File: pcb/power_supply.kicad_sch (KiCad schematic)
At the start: 16 parts, among them IC1 TLV76150DCYR, IC2 LM3940IMP-3.3_NOPB, J1 Jack-DC

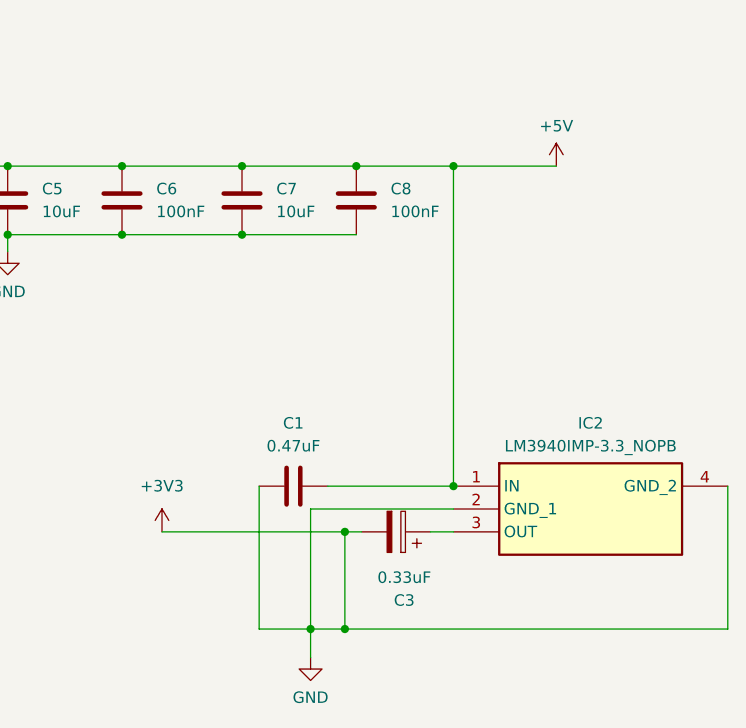
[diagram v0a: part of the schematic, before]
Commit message: a lot of audio finished, now onto ui
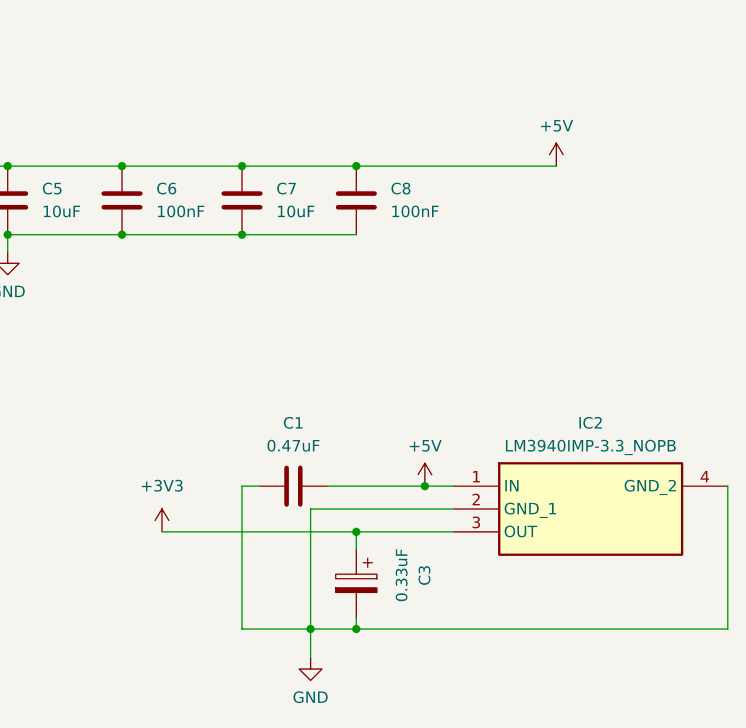
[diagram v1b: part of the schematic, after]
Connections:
- net +3V3: now also C3.1, IC2.3 (OUT); no longer C1.1, C2.2, C3.2, C4.2, C5.2, C6.2, C64.2, C65.2, C66.2, C67.2, C7.2, C8.2, IC1.1 (GND), IC2.2 (GND_1), IC2.4 (GND_2), J1.2
- new net GND: C1.1, C2.2, C3.2, C4.2, C5.2, C6.2, C64.2, C65.2, C66.2, C67.2, C7.2, C8.2, IC1.1 (GND), IC2.2 (GND_1), IC2.4 (GND_2), J1.2
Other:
- moved on the sheet: C3
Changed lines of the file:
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@@
   (junction (at 92.71 100.965) (diameter 0) (color 0 0 0 0)
   )
-  (junction (at 193.04 107.315) (diameter 0) (color 0 0 0 0)
-  )
-  (junction (at 205.105 55.88) (diameter 0) (color 0 0 0 0)
-  )
   (junction (at 92.71 50.8) (diameter 0) (color 0 0 0 0)
   )
@@
   (junction (at 189.23 107.315) (diameter 0) (color 0 0 0 0)
   )
+  (junction (at 194.31 107.315) (diameter 0) (color 0 0 0 0)
+  )
   (junction (at 181.61 55.88) (diameter 0) (color 0 0 0 0)
   )
@@
   (junction (at 80.01 93.345) (diameter 0) (color 0 0 0 0)
   )
-  (junction (at 193.04 96.52) (diameter 0) (color 0 0 0 0)
-  )
   (junction (at 155.575 63.5) (diameter 0) (color 0 0 0 0)
   )
   (junction (at 168.275 63.5) (diameter 0) (color 0 0 0 0)
   )
-  (junction (at 205.105 91.44) (diameter 0) (color 0 0 0 0)
-  )
   (junction (at 102.235 50.8) (diameter 0) (color 0 0 0 0)
   )
@@
   (junction (at 102.235 39.37) (diameter 0) (color 0 0 0 0)
   )
+  (junction (at 201.93 91.44) (diameter 0) (color 0 0 0 0)
+  )
+  (junction (at 194.31 96.52) (diameter 0) (color 0 0 0 0)
+  )
   (junction (at 155.575 55.88) (diameter 0) (color 0 0 0 0)
   )
@@
     (stroke (width 0) (type default))
   )
-  (wire (pts (xy 183.515 107.315) (xy 189.23 107.315))
+  (wire (pts (xy 172.72 96.52) (xy 194.31 96.52))
+    (stroke (width 0) (type default))
+  )
+  (wire (pts (xy 181.61 107.315) (xy 189.23 107.315))
     (stroke (width 0) (type default))
   )
@@
     (stroke (width 0) (type default))
   )
-  (wire (pts (xy 172.72 96.52) (xy 193.04 96.52))
-    (stroke (width 0) (type default))
-  )
-  (wire (pts (xy 191.135 91.44) (xy 205.105 91.44))
+  (wire (pts (xy 191.135 91.44) (xy 201.93 91.44))
     (stroke (width 0) (type default))
   )
@@
     (stroke (width 0) (type default))
   )
-  (wire (pts (xy 202.565 96.52) (xy 205.105 96.52))
+  (wire (pts (xy 201.93 91.44) (xy 205.105 91.44))
     (stroke (width 0) (type default))
   )
@@
     (stroke (width 0) (type default))
   )
-  (wire (pts (xy 189.23 107.315) (xy 193.04 107.315))
-    (stroke (width 0) (type default))
-  )
   (wire (pts (xy 80.01 93.345) (xy 92.71 93.345))
     (stroke (width 0) (type default))
@@
     (stroke (width 0) (type default))
   )
+  (wire (pts (xy 194.31 106.045) (xy 194.31 107.315))
+    (stroke (width 0) (type default))
+  )
   (wire (pts (xy 92.71 100.965) (xy 106.045 100.965))
     (stroke (width 0) (type default))
@@
     (stroke (width 0) (type default))
   )
+  (wire (pts (xy 194.31 107.315) (xy 235.585 107.315))
+    (stroke (width 0) (type default))
+  )
   (wire (pts (xy 235.585 91.44) (xy 235.585 107.315))
     (stroke (width 0) (type default))
   )
+  (wire (pts (xy 205.105 96.52) (xy 194.31 96.52))
+    (stroke (width 0) (type default))
+  )
   (wire (pts (xy 106.045 93.345) (xy 118.745 93.345))
     (stroke (width 0) (type default))
   )
-  (wire (pts (xy 194.945 96.52) (xy 193.04 96.52))
-    (stroke (width 0) (type default))
-  )
   (wire (pts (xy 66.675 55.88) (xy 69.85 55.88))
     (stroke (width 0) (type default))
   )
-  (wire (pts (xy 194.31 55.88) (xy 205.105 55.88))
+  (wire (pts (xy 194.31 55.88) (xy 216.535 55.88))
+    (stroke (width 0) (type default))
+  )
+  (wire (pts (xy 92.71 93.345) (xy 106.045 93.345))
+    (stroke (width 0) (type default))
+  )
+  (wire (pts (xy 80.01 100.965) (xy 80.01 102.87))
+    (stroke (width 0) (type default))
+  )
+  (wire (pts (xy 92.71 52.705) (xy 92.71 50.8))
+    (stroke (width 0) (type default))
+  )
+  (wire (pts (xy 181.61 63.5) (xy 194.31 63.5))
+    (stroke (width 0) (type default))
+  )
+  (wire (pts (xy 181.61 91.44) (xy 181.61 107.315))
+    (stroke (width 0) (type default))
+  )
+  (wire (pts (xy 102.235 55.88) (xy 102.235 66.675))
+    (stroke (width 0) (type default))
+  )
+  (wire (pts (xy 189.23 107.315) (xy 189.23 110.49))
+    (stroke (width 0) (type default))
+  )
+  (wire (pts (xy 98.425 39.37) (xy 102.235 39.37))
+    (stroke (width 0) (type default))
+  )
+  (wire (pts (xy 168.275 55.88) (xy 181.61 55.88))
+    (stroke (width 0) (type default))
+  )
+  (wire (pts (xy 102.235 48.26) (xy 102.235 50.8))
+    (stroke (width 0) (type default))
+  )
+  (wire (pts (xy 92.71 50.8) (xy 102.235 50.8))
+    (stroke (width 0) (type default))
+  )
+  (wire (pts (xy 135.89 57.785) (xy 135.89 55.88))
     (stroke (width 0) (type default))
   )
@@
     (stroke (width 0) (type default))
   )
-  (wire (pts (xy 92.71 93.345) (xy 106.045 93.345))
-    (stroke (width 0) (type default))
-  )
-  (wire (pts (xy 80.01 100.965) (xy 80.01 102.87))
-    (stroke (width 0) (type default))
-  )
-  (wire (pts (xy 92.71 52.705) (xy 92.71 50.8))
-    (stroke (width 0) (type default))
-  )
-  (wire (pts (xy 181.61 63.5) (xy 194.31 63.5))
-    (stroke (width 0) (type default))
-  )
-  (wire (pts (xy 183.515 91.44) (xy 183.515 107.315))
-    (stroke (width 0) (type default))
-  )
-  (wire (pts (xy 102.235 55.88) (xy 102.235 66.675))
-    (stroke (width 0) (type default))
-  )
-  (wire (pts (xy 189.23 107.315) (xy 189.23 110.49))
-    (stroke (width 0) (type default))
-  )
-  (wire (pts (xy 98.425 39.37) (xy 102.235 39.37))
-    (stroke (width 0) (type default))
-  )
-  (wire (pts (xy 168.275 55.88) (xy 181.61 55.88))
-    (stroke (width 0) (type default))
-  )
-  (wire (pts (xy 102.235 48.26) (xy 102.235 50.8))
-    (stroke (width 0) (type default))
-  )
-  (wire (pts (xy 92.71 50.8) (xy 102.235 50.8))
-    (stroke (width 0) (type default))
-  )
-  (wire (pts (xy 135.89 57.785) (xy 135.89 55.88))
-    (stroke (width 0) (type default))
-  )
   (wire (pts (xy 168.275 63.5) (xy 181.61 63.5))
     (stroke (width 0) (type default))
@@
     (stroke (width 0) (type default))
   )
-  (wire (pts (xy 193.04 107.315) (xy 235.585 107.315))
-    (stroke (width 0) (type default))
-  )
-  (wire (pts (xy 205.105 55.88) (xy 205.105 91.44))
+  (wire (pts (xy 189.23 107.315) (xy 194.31 107.315))
+    (stroke (width 0) (type default))
+  )
+  (wire (pts (xy 181.61 91.44) (xy 183.515 91.44))
+    (stroke (width 0) (type default))
+  )
+  (wire (pts (xy 194.31 96.52) (xy 194.31 98.425))
     (stroke (width 0) (type default))
   )
   (wire (pts (xy 155.575 63.5) (xy 168.275 63.5))
-    (stroke (width 0) (type default))
-  )
-  (wire (pts (xy 193.04 96.52) (xy 193.04 107.315))
-    (stroke (width 0) (type default))
-  )
-  (wire (pts (xy 205.105 55.88) (xy 216.535 55.88))
     (stroke (width 0) (type default))
   )
@@
         (path "/eb787481-08cd-41a4-a128-173fa6227c32/4ec3bf5a-5f62-4a58-b8f9-e874725801fb"
           (reference "C8") (unit 1)
+        )
+      )
+    )
+  )
+  (symbol (lib_id "power:+5V") (at 201.93 91.44 0) (unit 1)
+    (in_bom yes) (on_board yes) (dnp no) (fields_autoplaced)
+    (property "Reference" "#PWR0123" (at 201.93 95.25 0)
+      (effects (font (size 1.27 1.27)) hide)
+    )
+    (property "Value" "+5V" (at 201.93 86.995 0)
+      (effects (font (size 1.27 1.27)))
+    )
+    (property "Footprint" "" (at 201.93 91.44 0)
+      (effects (font (size 1.27 1.27)) hide)
+    )
+    (property "Datasheet" "" (at 201.93 91.44 0)
+      (effects (font (size 1.27 1.27)) hide)
+    )
+    (pin "1")
+    (instances
+      (project "bt_pcb"
+        (path "/eb787481-08cd-41a4-a128-173fa6227c32/4ec3bf5a-5f62-4a58-b8f9-e874725801fb"
+          (reference "#PWR0123") (unit 1)
         )
       )
@@
     )
   )
-  (symbol (lib_id "Device:C_Polarized") (at 198.755 96.52 270) (mirror x) (unit 1)
+  (symbol (lib_id "Device:C_Polarized") (at 194.31 102.235 0) (mirror y) (unit 1)
     (in_bom yes) (on_board yes) (dnp no)
-    (property "Reference" "C3" (at 199.644 104.14 90)
-      (effects (font (size 1.27 1.27)))
-    )
-    (property "Value" "0.33uF" (at 199.644 101.6 90)
-      (effects (font (size 1.27 1.27)))
-    )
-    (property "Footprint" "" (at 194.945 95.5548 0)
-      (effects (font (size 1.27 1.27)) hide)
-    )
-    (property "Datasheet" "~" (at 198.755 96.52 0)
-      (effects (font (size 1.27 1.27)) hide)
-    )
+    (property "Reference" "C3" (at 201.93 101.346 90)
+      (effects (font (size 1.27 1.27)))
+    )
+    (property "Value" "0.33uF" (at 199.39 101.346 90)
+      (effects (font (size 1.27 1.27)))
+    )
+    (property "Footprint" "" (at 193.3448 106.045 0)
+      (effects (font (size 1.27 1.27)) hide)
+    )
+    (property "Datasheet" "~" (at 194.31 102.235 0)
+      (effects (font (size 1.27 1.27)) hide)
+    )
